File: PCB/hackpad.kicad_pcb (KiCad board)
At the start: 2 copper layers, 49 x 85.1 mm, 12 parts, among them J1 Conn_01x04, SW1 SW_Push, SW2 SW_Push, SW3 SW_Push, SW4 SW_Push, U1 XIAO-RP2040-DIP

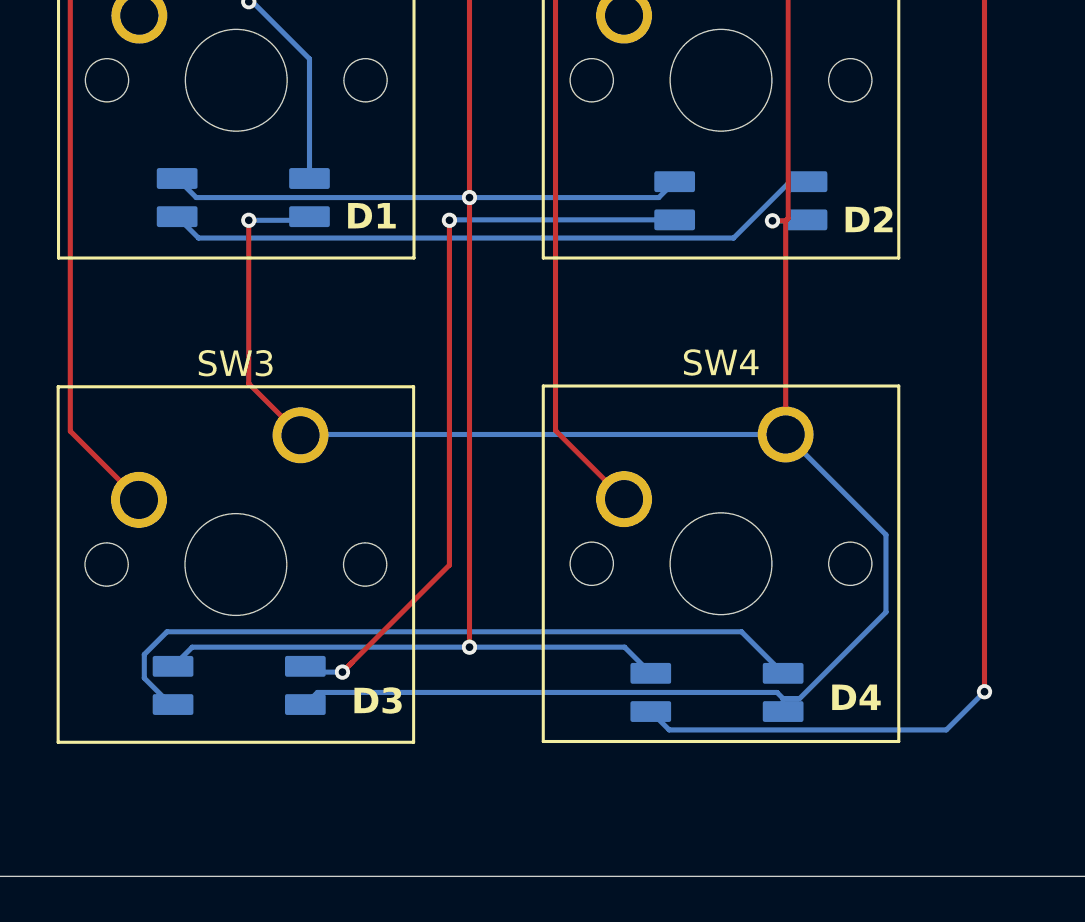
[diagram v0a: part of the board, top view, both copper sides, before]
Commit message: Refactor code structure for improved readability and maintainability
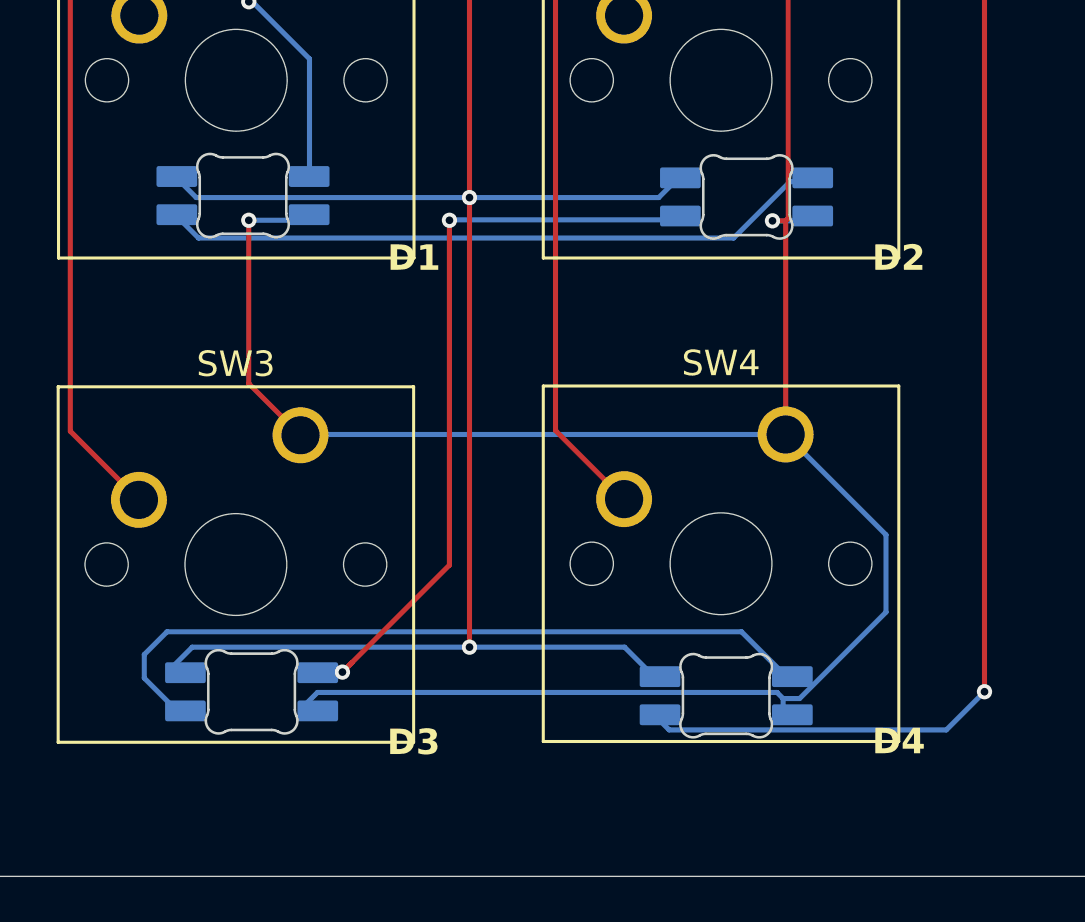
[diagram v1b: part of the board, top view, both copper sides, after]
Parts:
- moved D3 0.55 mm to (143.0, 129.1)
- moved D4 0.38 mm to (161.6, 129.3)
- moved D2 0.27 mm to (162.4, 109.7)
- moved D1 0.08 mm to (142.7, 109.6)

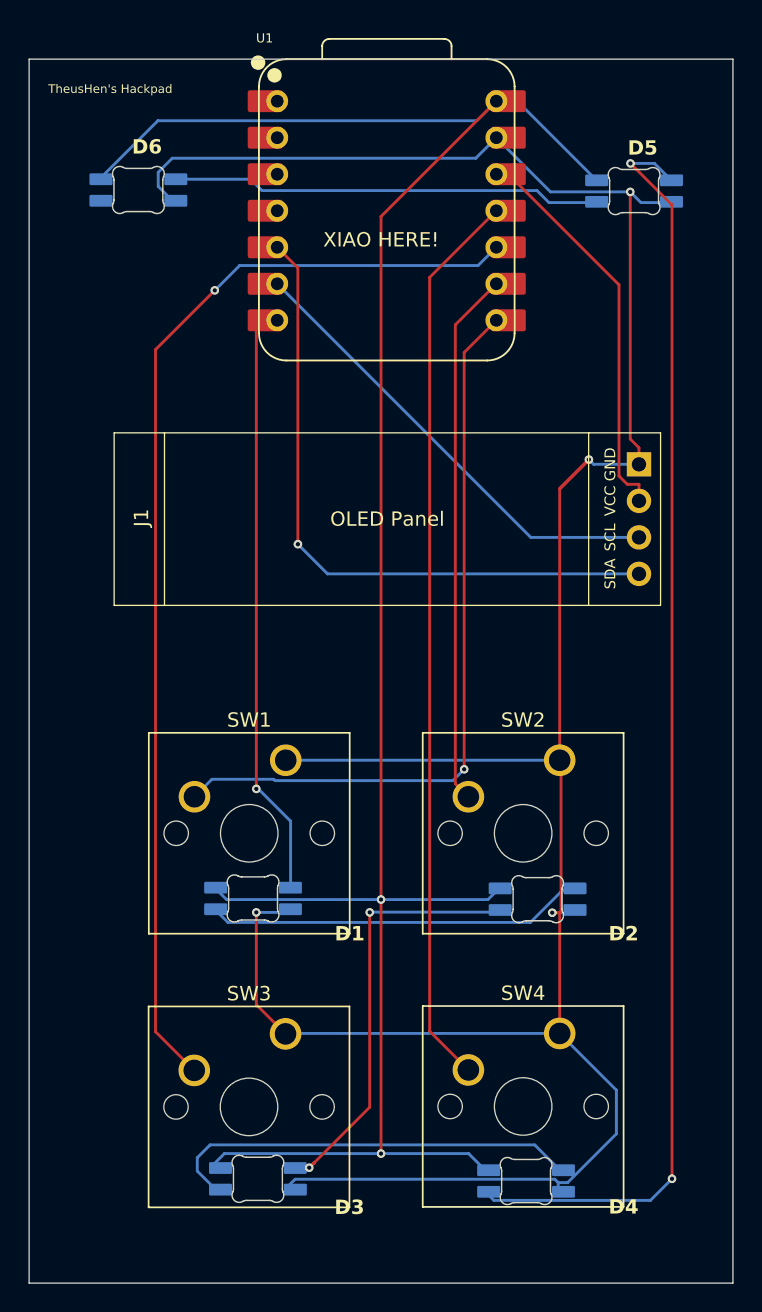
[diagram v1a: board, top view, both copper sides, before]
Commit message: Refactor code structure for improved readability and maintainability
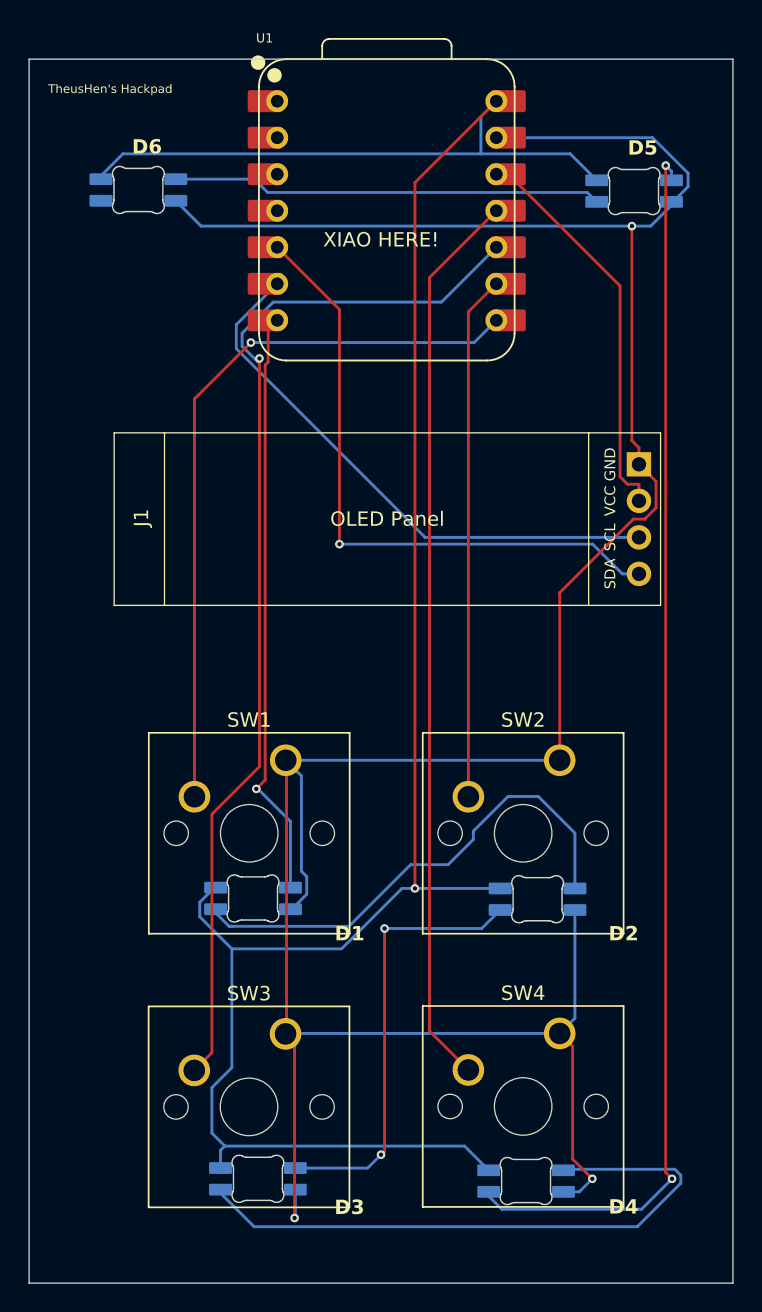
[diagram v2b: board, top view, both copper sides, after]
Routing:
- net Net-(D3-DOUT): track 28.6 -> 43.4 mm
- net Net-(D1-DOUT): track 26.0 -> 34.6 mm
- net I2C_SCL: track 33.3 -> 40.0 mm
- net Net-(U1-GPIO4/MISO): track 78.7 -> 75.2 mm
- net +5V: track 156.2 -> 159.6 mm, vias 2 -> 1
- net Net-(D4-DOUT): track 89.2 -> 86.1 mm
- net I2C_SDA: track 46.7 -> 45.0 mm
- net GND: track 202.5 -> 201.1 mm, vias 4 -> 3
- net Net-(D2-DOUT): track 32.1 -> 30.8 mm
- net Net-(U1-GPIO1/RX): track 52.6 -> 51.8 mm
- net Net-(U1-GPIO2/SCK): track 38.1 -> 37.3 mm
